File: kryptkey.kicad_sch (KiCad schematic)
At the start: 35 parts, among them J1 Conn_01x04_Pin, J2 Conn_01x04_Pin, P2 USB_C_Plug_USB2.0, SW1 SW_Push, SW2 SW_Push, SW3 SW_Push, SW4 SW_SPDT, U1 AMS1117-3.3, U2 STM32F103C8T6, Y1 16MHz

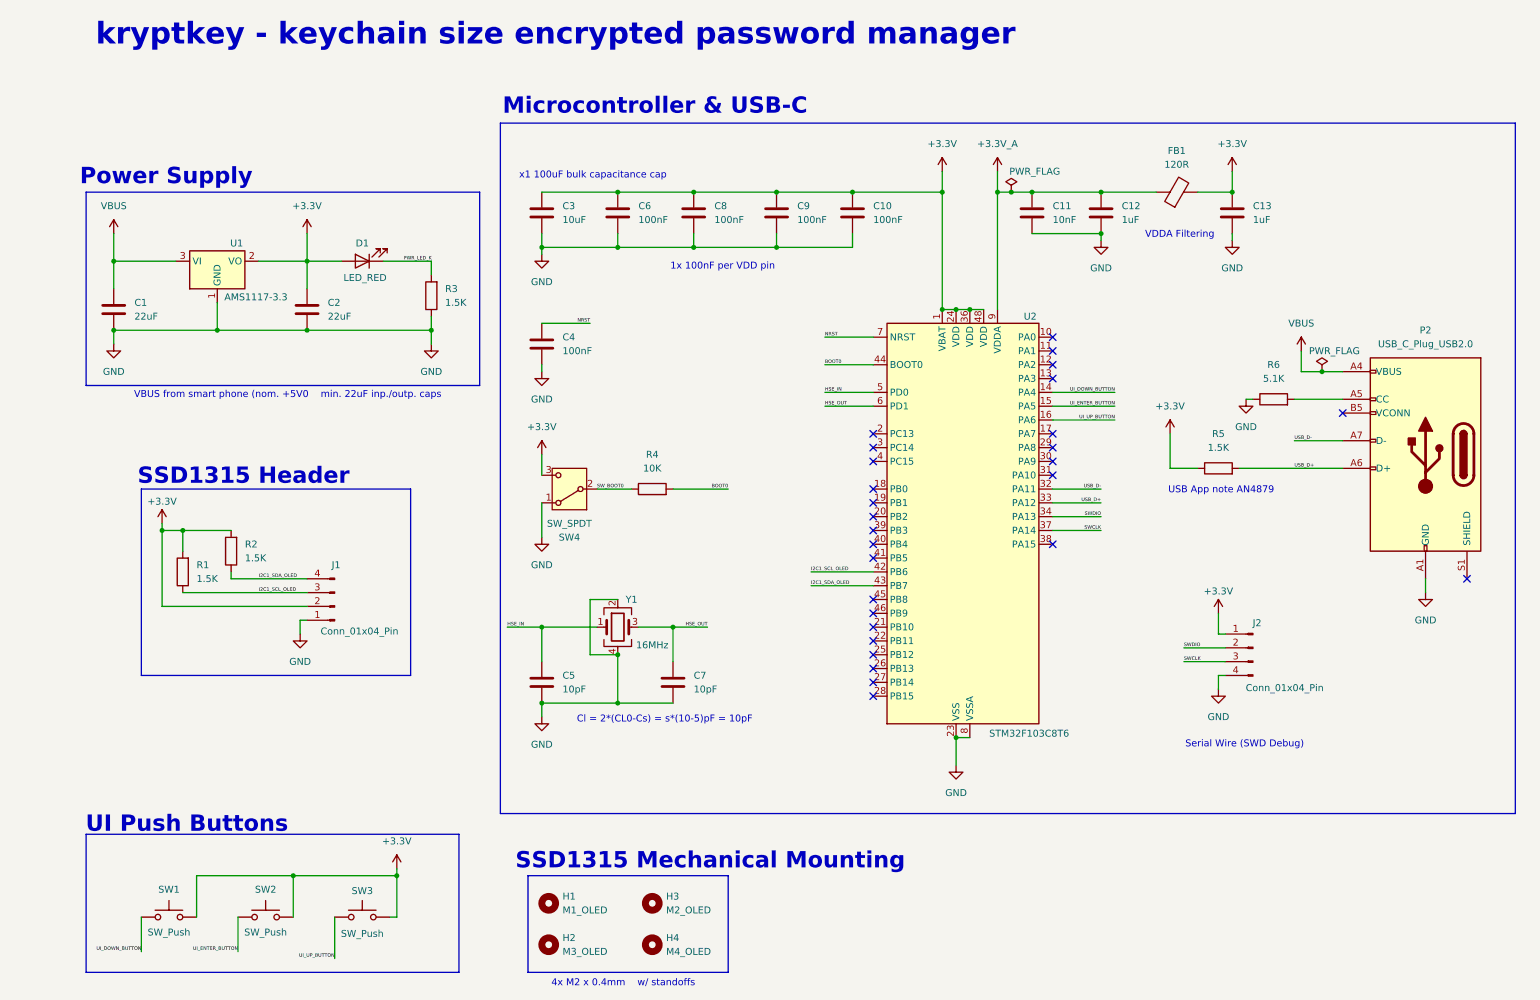
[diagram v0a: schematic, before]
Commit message: first pass routing
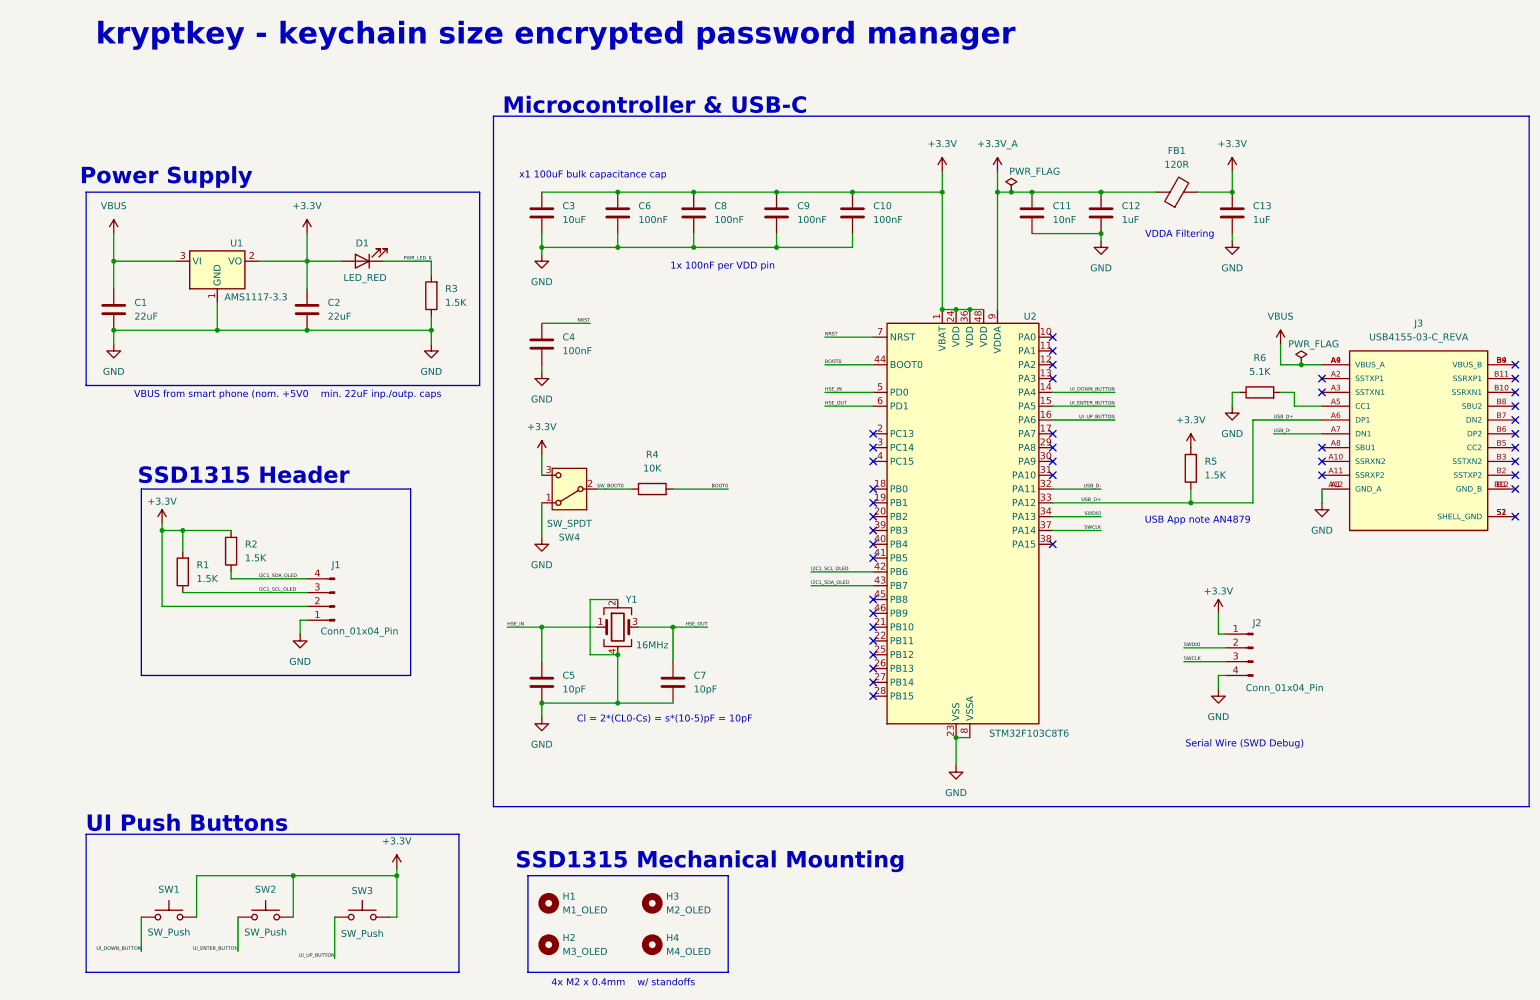
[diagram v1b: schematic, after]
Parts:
- removed P2: USB_C_Plug_USB2.0, Connector_USB:USB_C_Plug_ShenzhenJingTuoJin_918-118A2021Y40002_Vertical, symbol Connector:USB_C_Plug_USB2.0
- added J3: USB4155-03-C_REVA, USB4155-03-C_REVA:GCT_USB4155-03-C_REVA, symbol USB4155-03-C:USB4155-03-C_REVA
- FB1: footprint Inductor_SMD:L_12x12mm_H8mm -> Inductor_SMD:L_0603_1608Metric
- H1, H2, H3, H4: footprint MountingHole:MountingHole_2.5mm -> MountingHole:MountingHole_2.7mm_M2.5
- J2: footprint Connector_PinHeader_2.54mm:PinHeader_1x04_P2.54mm_Vertical -> Connector_PinHeader_2.54mm:PinHeader_1x04_P2.54mm_Horizontal
- SW4: footprint Button_Switch_THT:SW_E-Switch_EG1224_SPDT_Angled -> Button_Switch_THT:SW_E-Switch_EG1271_SPDT
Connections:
- net +3.3V: now also R5.2; no longer R5.1
- net GND: now also J3.A1 (GND_A), J3.A12 (GND_A)
- net USB_D+: now also R5.1, J3.A6 (DP1); no longer R5.2
- net USB_D-: now also J3.A7 (DN1)
- net VBUS: now also J3.A4 (VBUS_A), J3.A9 (VBUS_A)
- net at R6.2: now also J3.A5 (CC1)
- new net: J3.B1 (GND_B), J3.B12 (GND_B)
- new net: J3.B4 (VBUS_B), J3.B9 (VBUS_B)
- new net: J3.S1 (SHELL_GND), J3.S2 (SHELL_GND)
- no-connect marks 28 -> 42
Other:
- moved on the sheet: R5, R6
